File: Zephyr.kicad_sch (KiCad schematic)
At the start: 35 parts, among them J1 Conn_02x03_Counter_Clockwise, J11 Conn_01x03, J13 Conn_01x03, J14 Conn_01x06, Q1 MMBT3904, Q2 MMBT3904, SW4 SW_Push, U1 STM32F405RGT6, Y1 32.768KHz 12.5pF, Y2 8MHz 12pF

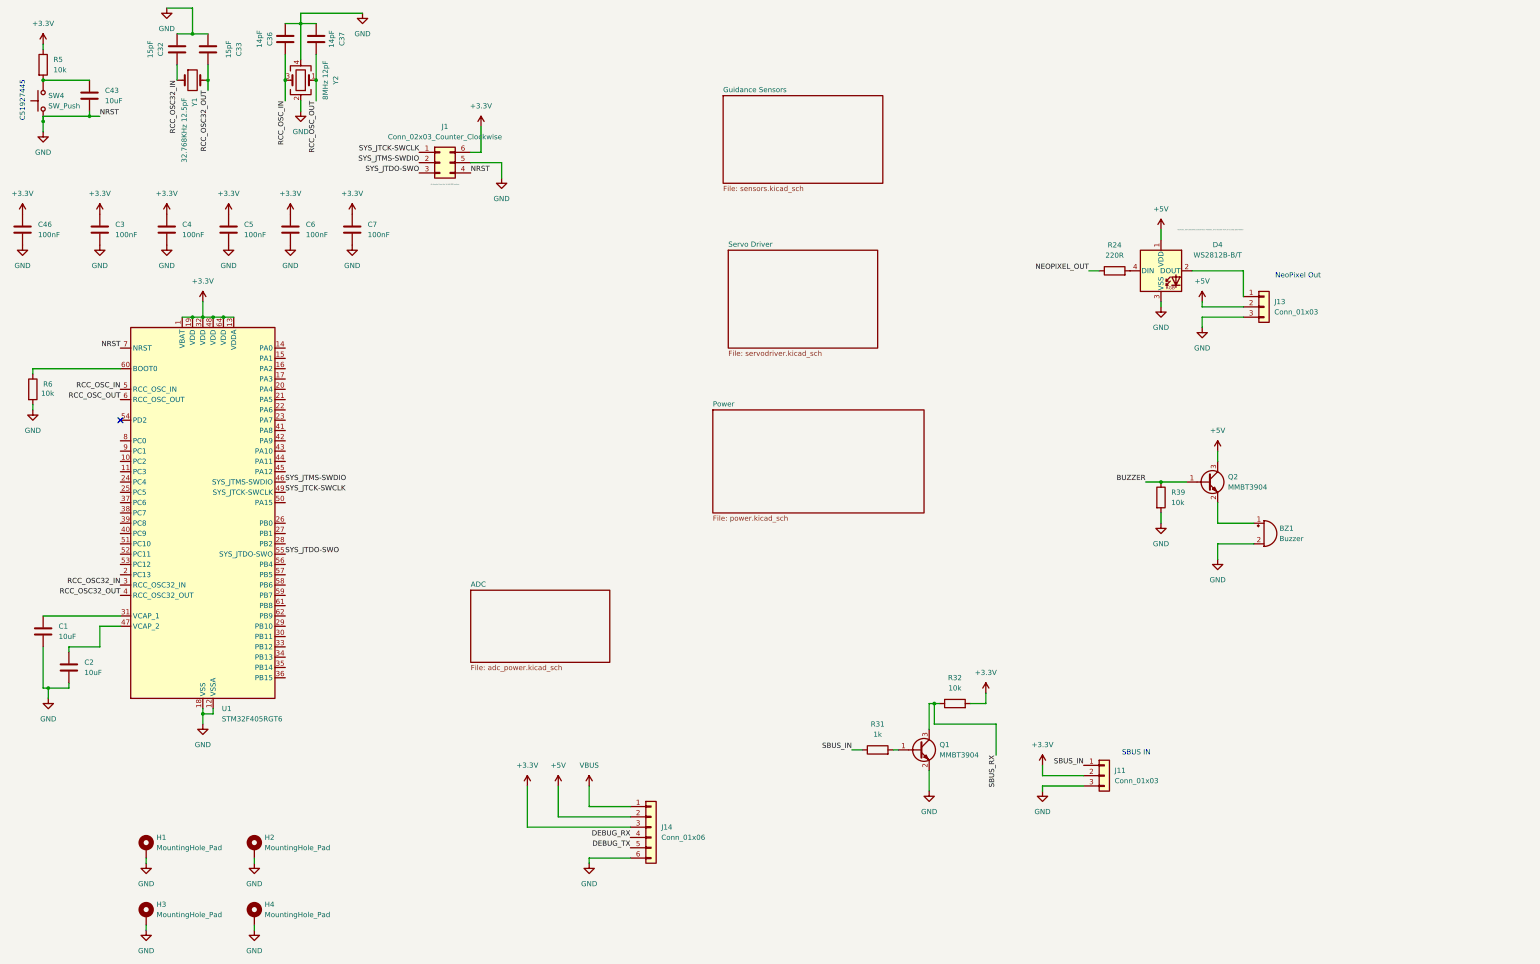
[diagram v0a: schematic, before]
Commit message: Work on power supply...
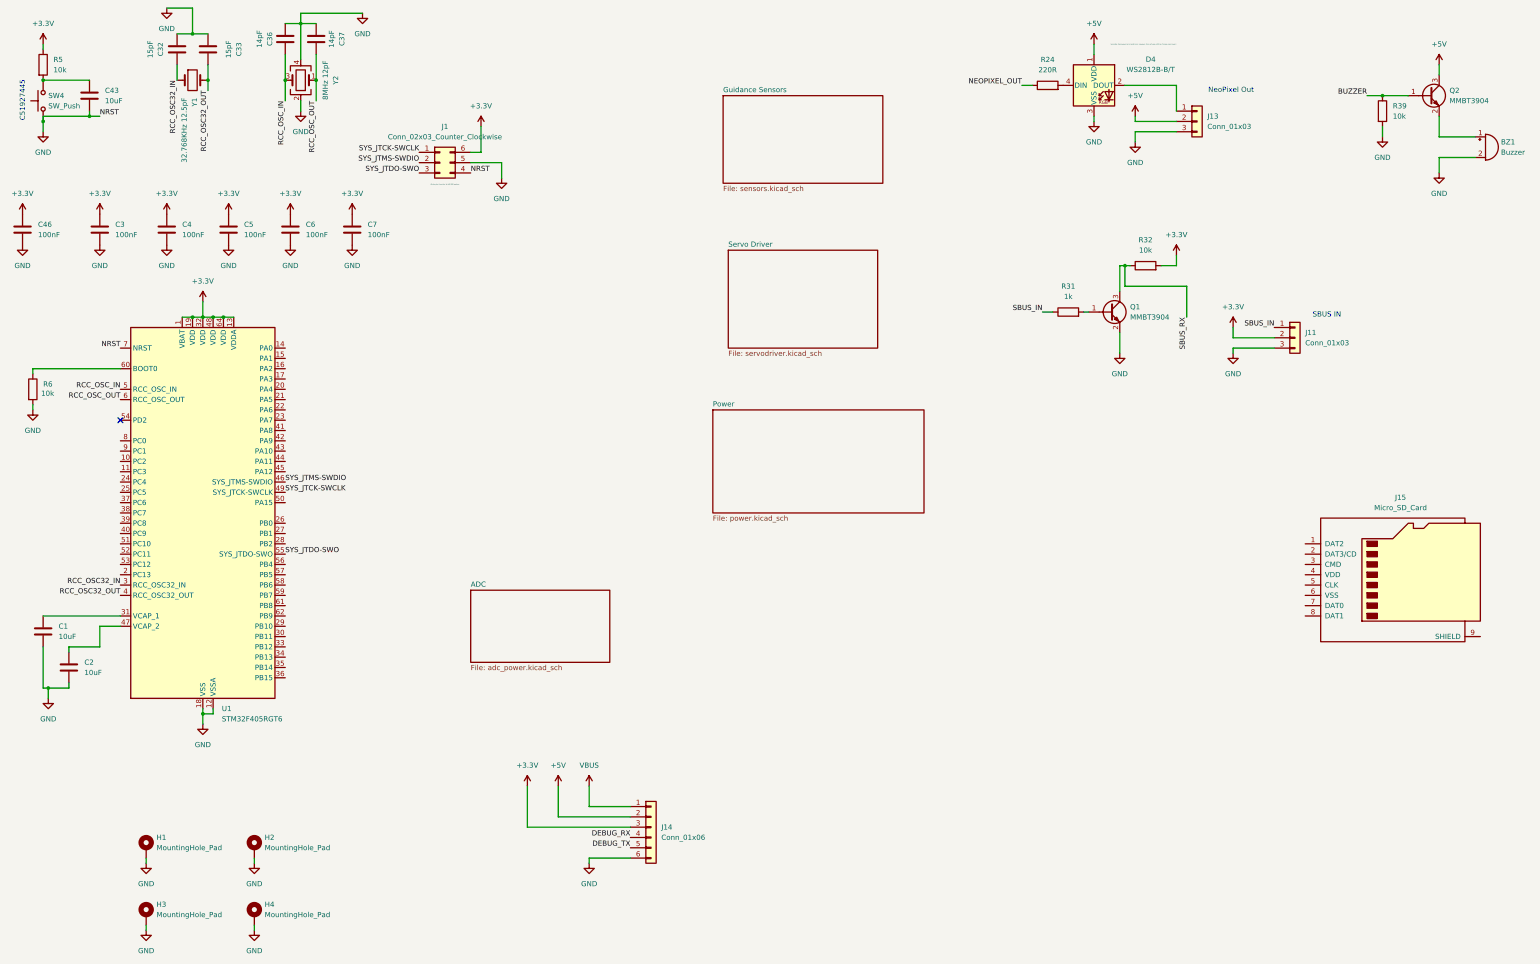
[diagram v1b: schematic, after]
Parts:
- added J15: Micro_SD_Card, symbol Connector:Micro_SD_Card
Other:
- moved on the sheet: BZ1, D4, J11, J13, Q1, Q2, R24, R31, R32, R39
